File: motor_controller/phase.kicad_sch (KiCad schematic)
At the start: 13 parts

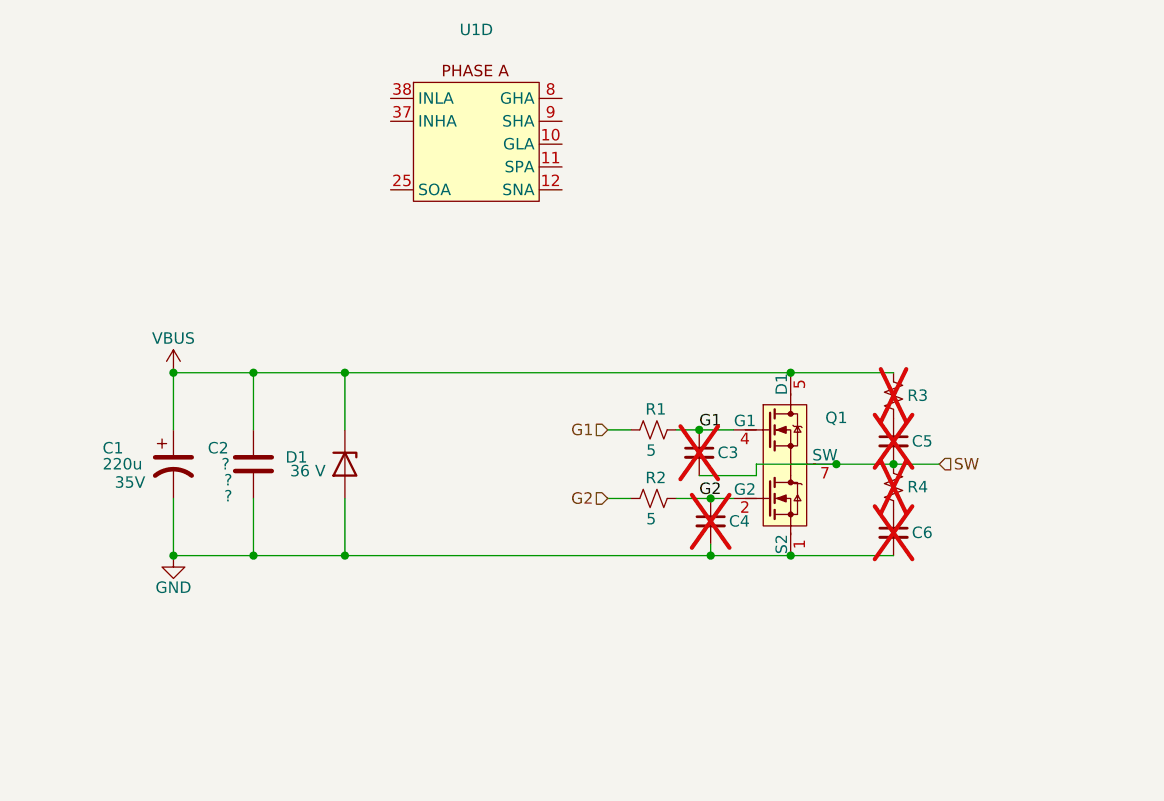
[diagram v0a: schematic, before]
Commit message: e
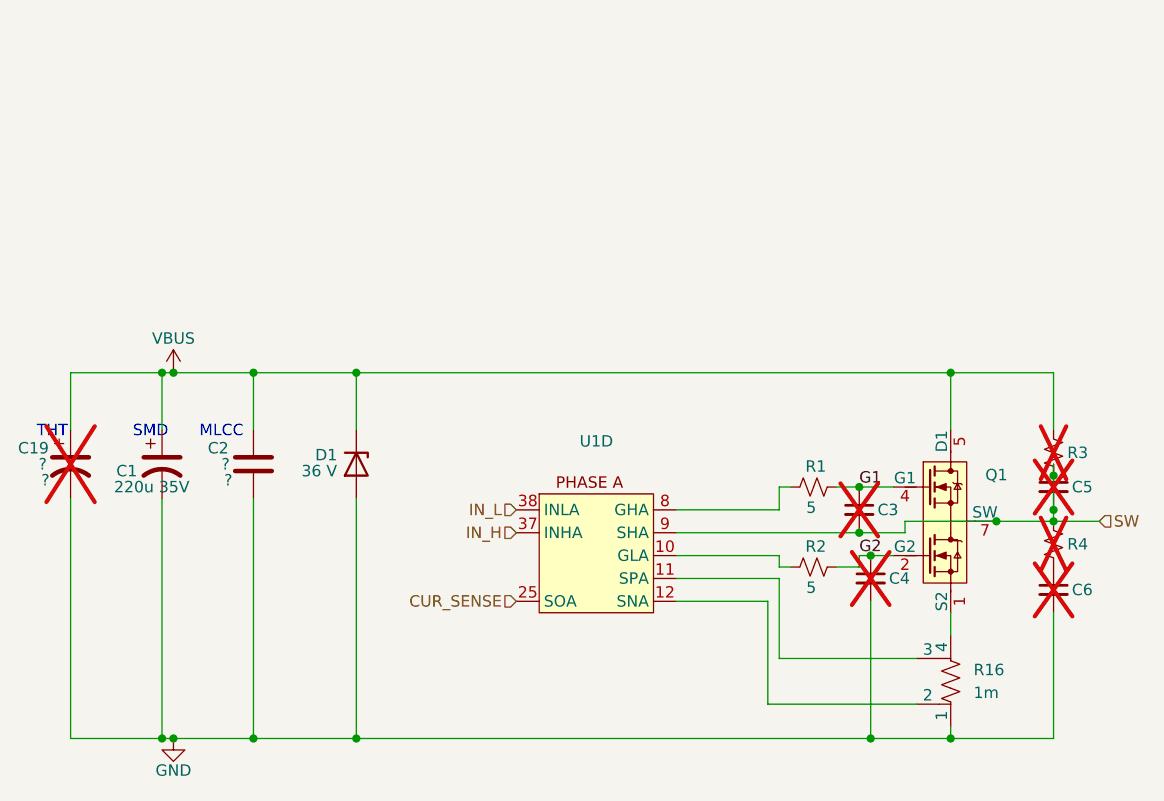
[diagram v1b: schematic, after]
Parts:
- added C19: ?, Capacitor_THT:C_Disc_D3.0mm_W1.6mm_P2.50mm, symbol Device:C_Polarized_US
- added R16: 1m, project:R_0805_SHUNT, symbol Device:R_Shunt_US
- C1: value 220u -> 220u 35V; Voltage 35V -> (none)
- U1: footprint (none) -> Package_DFN_QFN:VQFN-48-1EP_7x7mm_P0.5mm_EP4.1x4.1mm_ThermalVias
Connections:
- net G1: no longer R1.1
- net G2: no longer R2.1
- net GND: now also C19.2, R16.1; no longer Q1.1 (S2)
- net SW: now also C5.1, R3.2, U1.9 (SHA)
- net VBUS: now also C19.1
- net at U1.10 (GLA): now also R2.1
- net at U1.11 (SPA): now also R16.3
- net at U1.12 (SNA): now also R16.2
- net CUR_SENSE: now reaches U1.25 (SOA)
- net IN_H: now reaches U1.37 (INHA)
- net IN_L: now reaches U1.38 (INLA)
- net at U1.8 (GHA): now also R1.1
- new net: Q1.1 (S2), R16.4
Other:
- note added: "MLCC"
- note added: "SMD"
- note added: "THT"
- moved on the sheet: C1, C3, C4, C5, C6, D1, Q1, R1, R2, R3, R4, U1D

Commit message: BALLed out
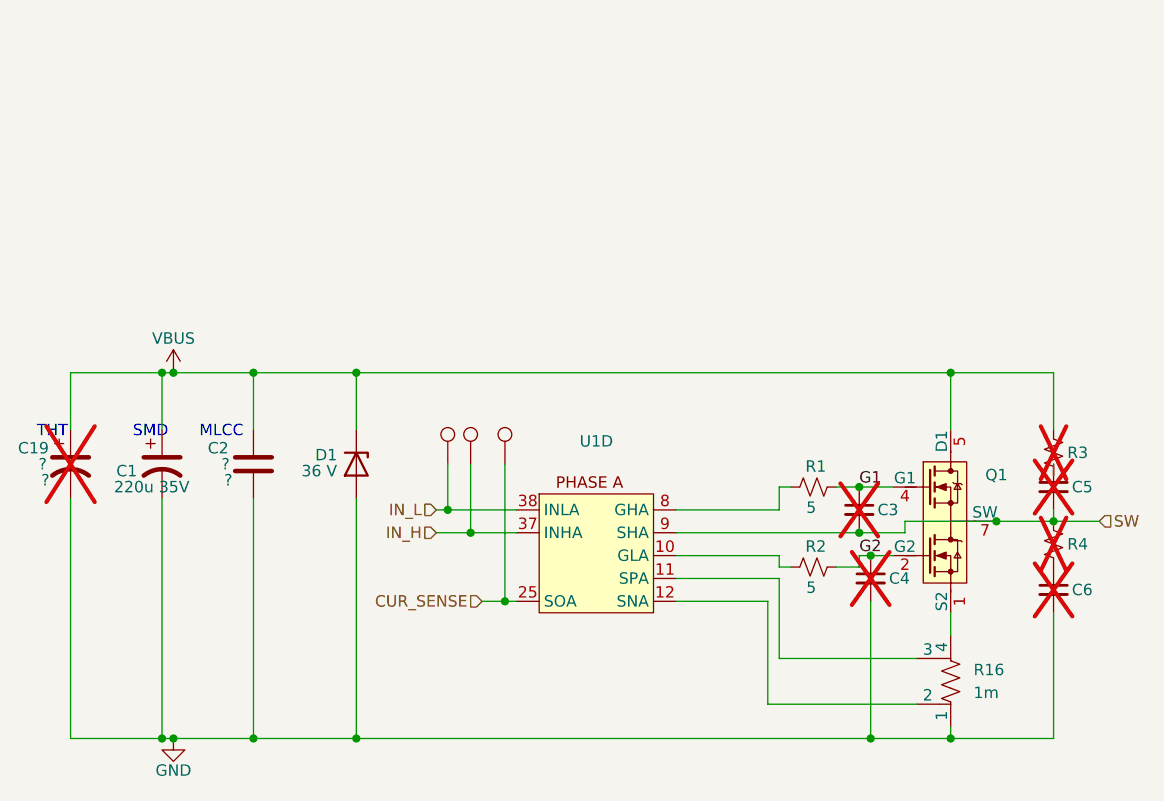
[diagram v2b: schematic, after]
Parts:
- added TP1, TP4, TP7: test point, project:test point d1.5, symbol project:TestPoint
- U1: footprint Package_DFN_QFN:VQFN-48-1EP_7x7mm_P0.5mm_EP4.1x4.1mm_ThermalVias -> (none)
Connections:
- net CUR_SENSE: now also TP7.1
- net IN_H: now also TP4.1
- net IN_L: now also TP1.1
- net SW: no longer C5.1, R3.2
- new net: C5.1, R3.2
